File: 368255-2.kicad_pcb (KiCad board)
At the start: 2 copper layers, 158 x 114 mm, 27 parts, among them J11 5569-08A2, J2 5569-18A2, J21 Conn_01x01_Pin, J22 Conn_01x01_Pin, J23 Conn_01x01_Pin, J24 Conn_01x01_Pin, J25 Conn_01x01_Pin, J26 Conn_01x01_Pin, J27 Conn_01x01_Pin, J28 Conn_01x01_Pin, J3 5569-06A2, J4 5569-16A2, J5 5569-20A2, P1 368255-2, U1 ULN2003A

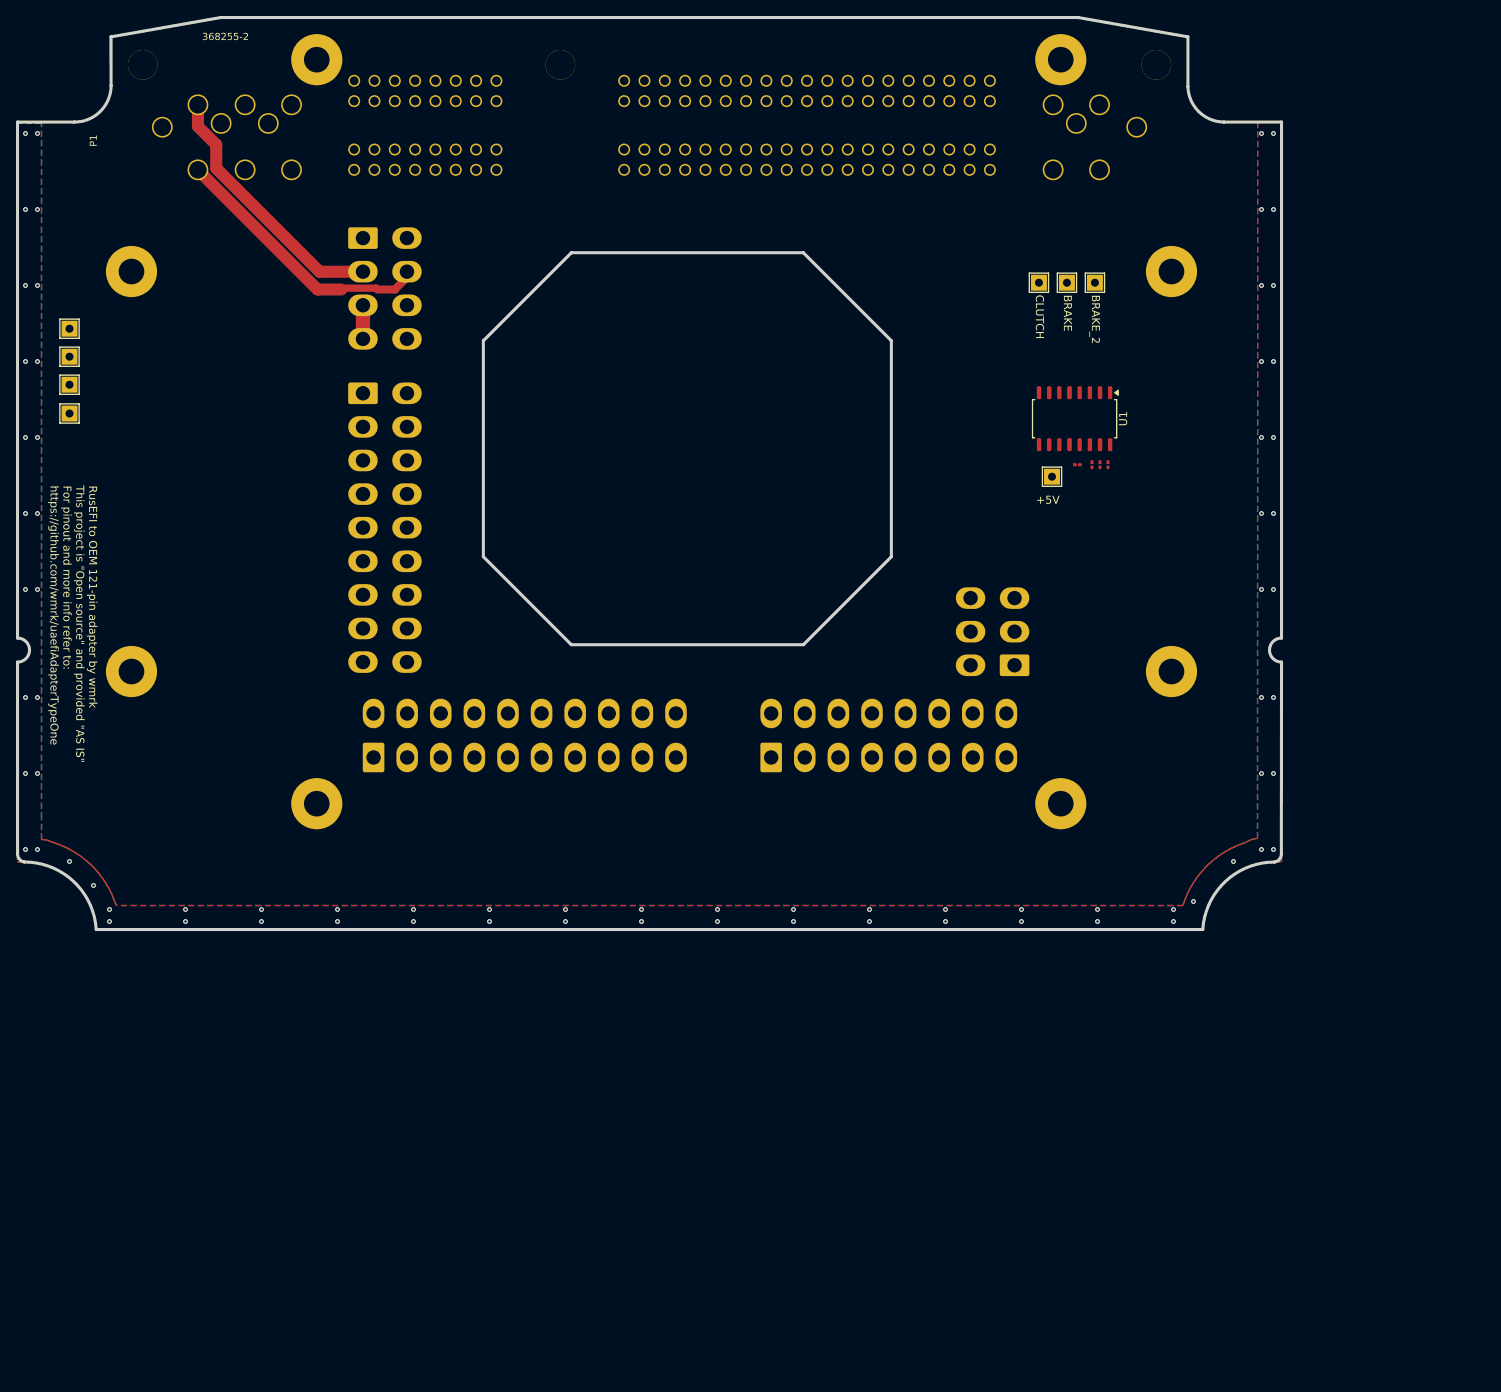
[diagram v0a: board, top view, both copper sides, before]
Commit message: tracing but not finished
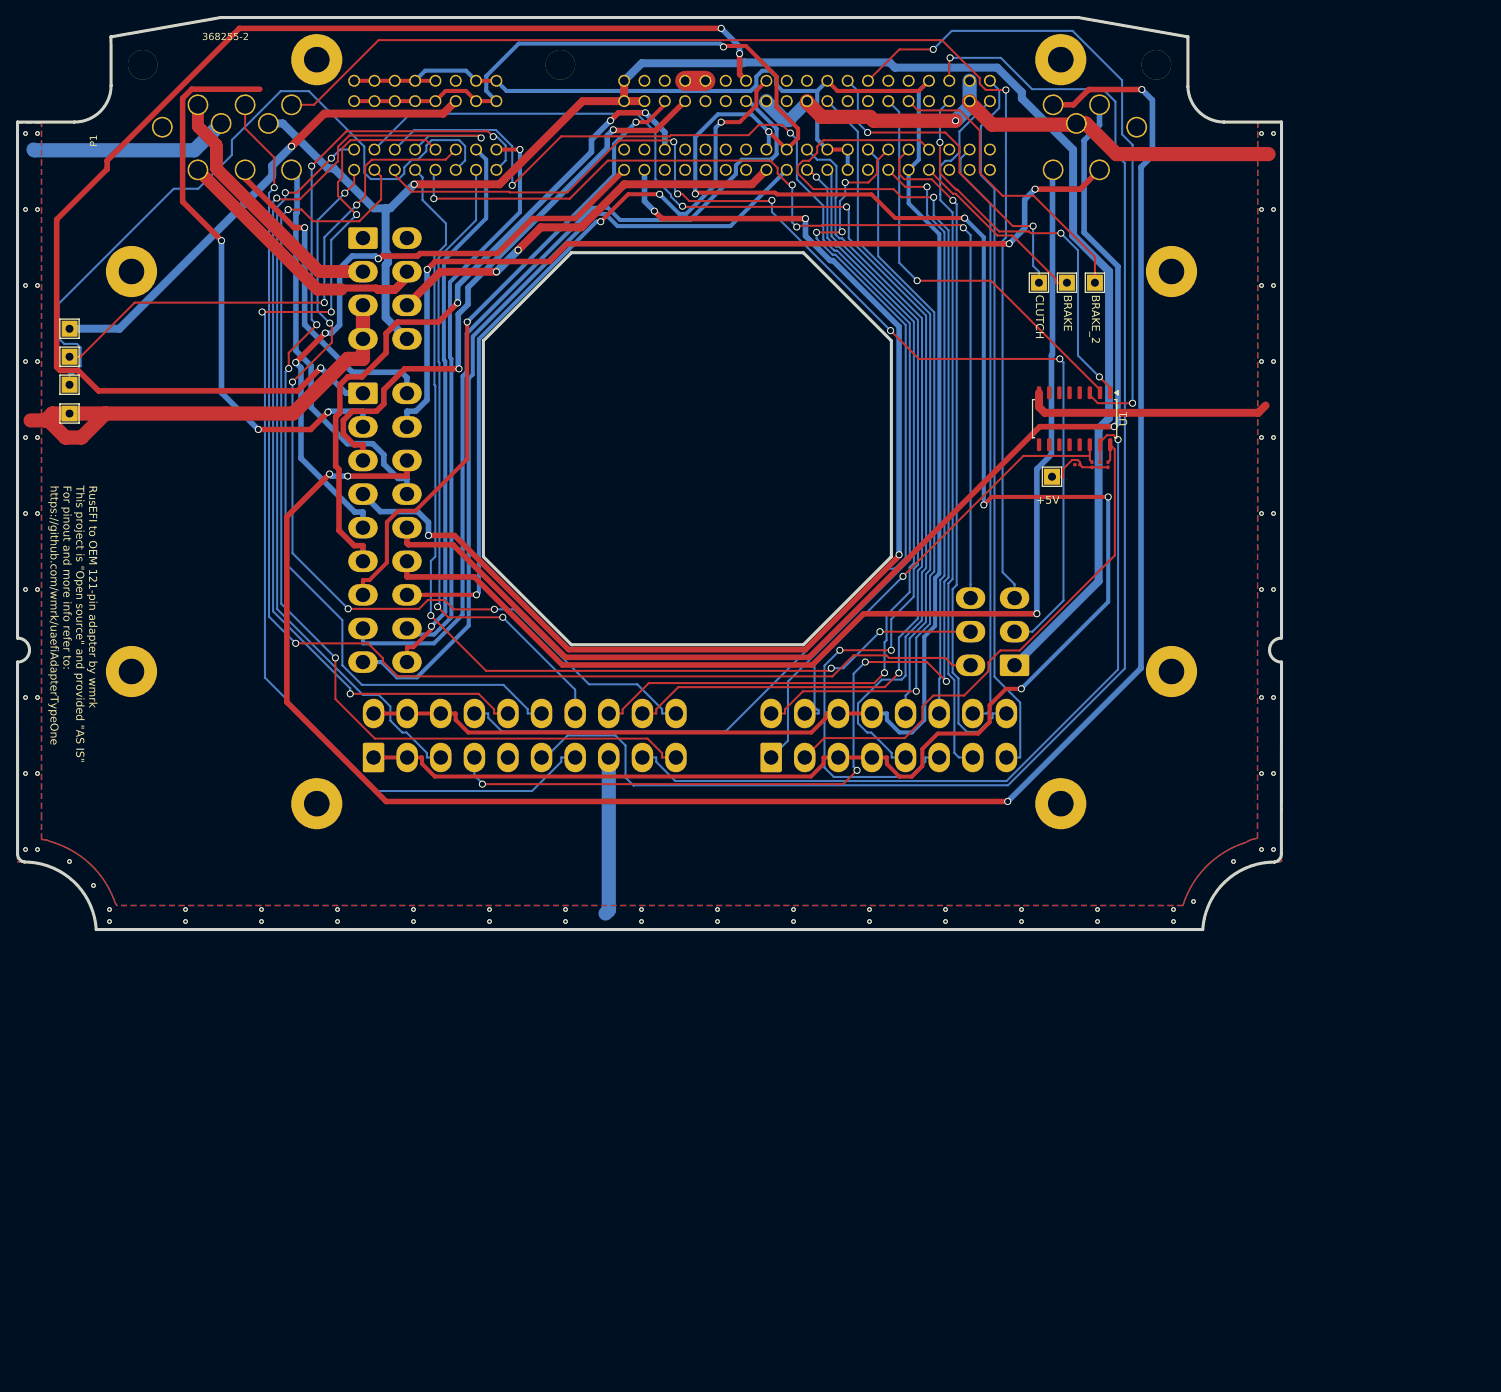
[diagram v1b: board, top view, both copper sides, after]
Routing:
- net +5VP: track 0.00 -> 305.7 mm, vias 0 -> 7
- net GNDA: track 0.00 -> 250.8 mm
- net /OUT_IGN3: track 0.00 -> 246.7 mm, vias 0 -> 4
- net +12V: track 0.00 -> 210.4 mm, vias 0 -> 1
- net GND: track 4.20 -> 209.3 mm, vias 74 -> 75
- net /IN_HALL2: track 0.00 -> 182.9 mm, vias 0 -> 1
- net /IN_PPS2: track 0.00 -> 176.2 mm, vias 0 -> 5
- net /OUT_INJ6: track 0.00 -> 161.9 mm, vias 0 -> 3
- net /3_WBO_Heater: track 0.00 -> 160.0 mm, vias 0 -> 1
- net /6_WBO_Un: track 0.00 -> 158.4 mm, vias 0 -> 2
- net /OUT_INJ3: track 0.00 -> 153.0 mm, vias 0 -> 4
- net /IN_AUX1_EWG_POS_SENSOR: track 0.00 -> 151.4 mm, vias 0 -> 2
- net /OUT_IGN2: track 0.00 -> 151.2 mm, vias 0 -> 1
- net /IN_FLEX: track 0.00 -> 151.0 mm, vias 0 -> 2
- net /OUT_IGN1: track 0.00 -> 144.2 mm, vias 0 -> 1
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
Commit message: refactoring
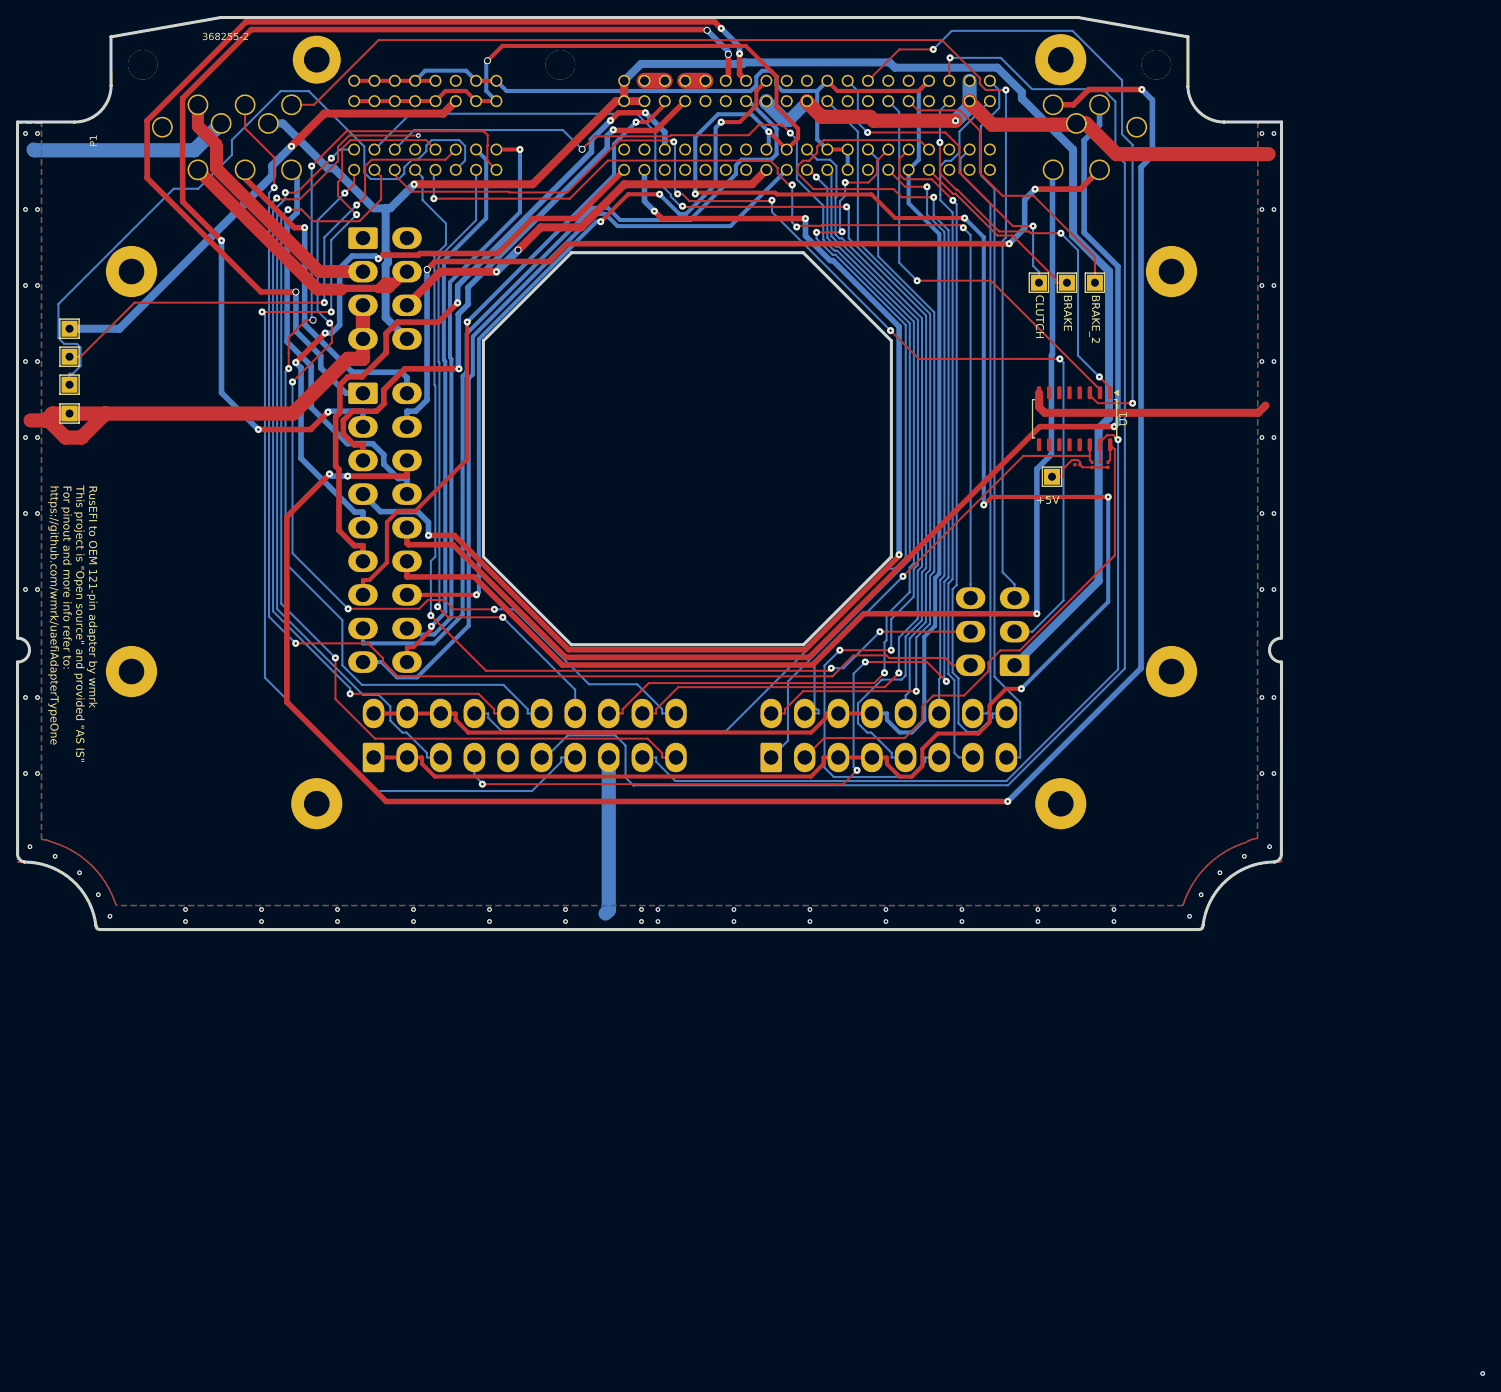
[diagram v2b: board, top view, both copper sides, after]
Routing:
- net /OUT_INJ5: track 71.4 -> 138.0 mm, vias 3 -> 5
- net /OUT_INJ6: track 161.9 -> 134.1 mm
- net /IN_AUX3_FUEL_PRESSURE_SENSOR: track 126.3 -> 109.3 mm
- net /IN_AUX1_EWG_POS_SENSOR: track 151.4 -> 144.8 mm
- net /OUT_DC1-: track 0.00 -> 2.54 mm
- net /VR_MAX9924+: track 125.3 -> 124.0 mm, vias 4 -> 3
- net /OUT_IGN5: track 49.1 -> 50.0 mm
- net +5VP: track 305.7 -> 306.4 mm
- net (no net): vias 0 -> 1
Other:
- outline, holes or cut-outs redrawn
